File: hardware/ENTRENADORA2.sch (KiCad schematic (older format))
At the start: 74 parts

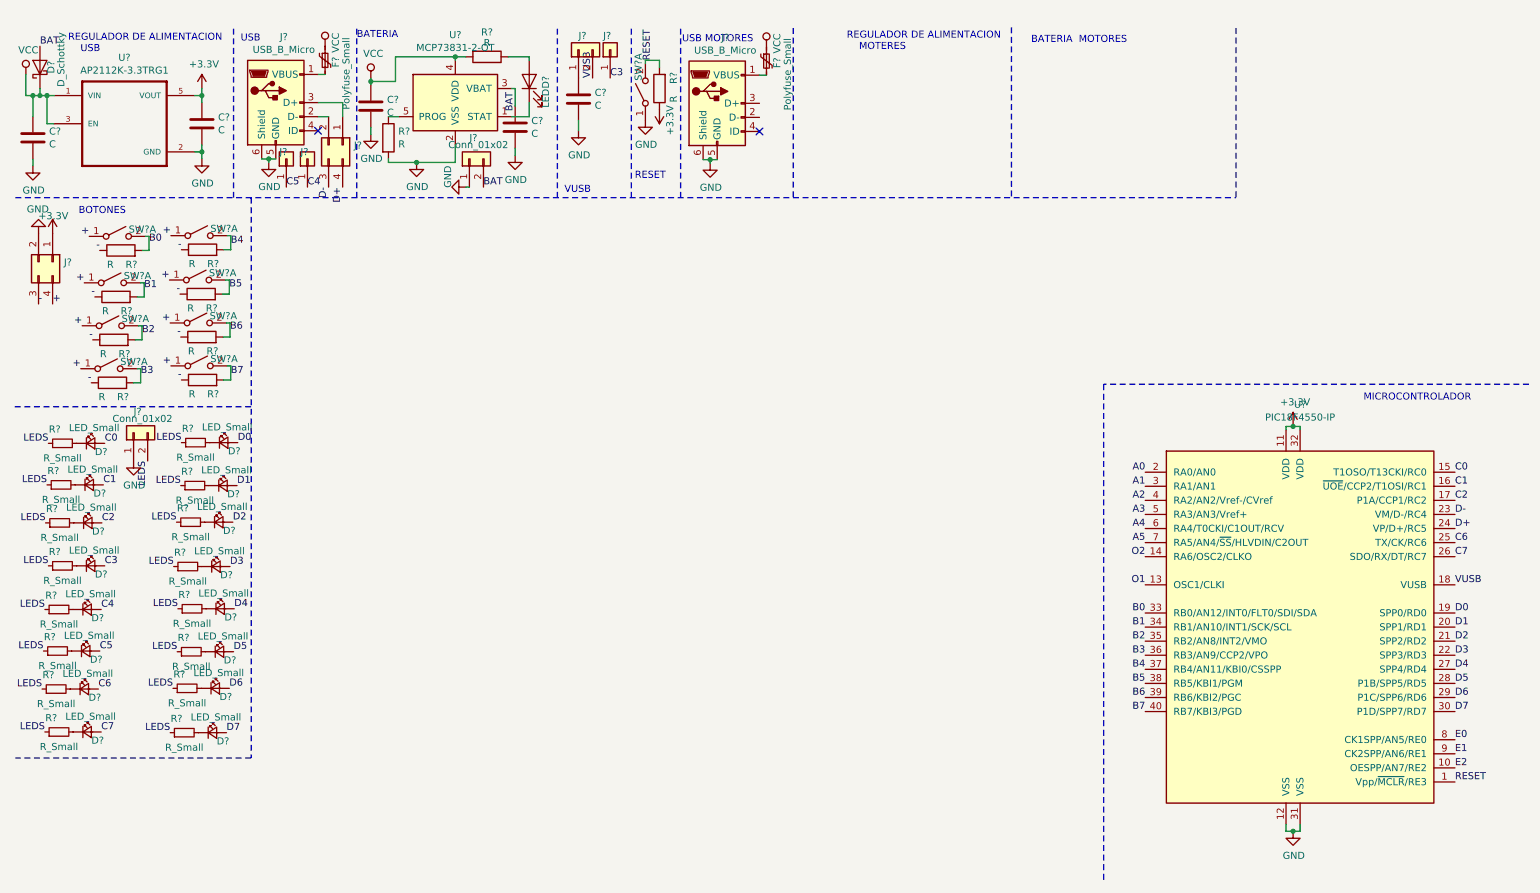
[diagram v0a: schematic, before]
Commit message: co
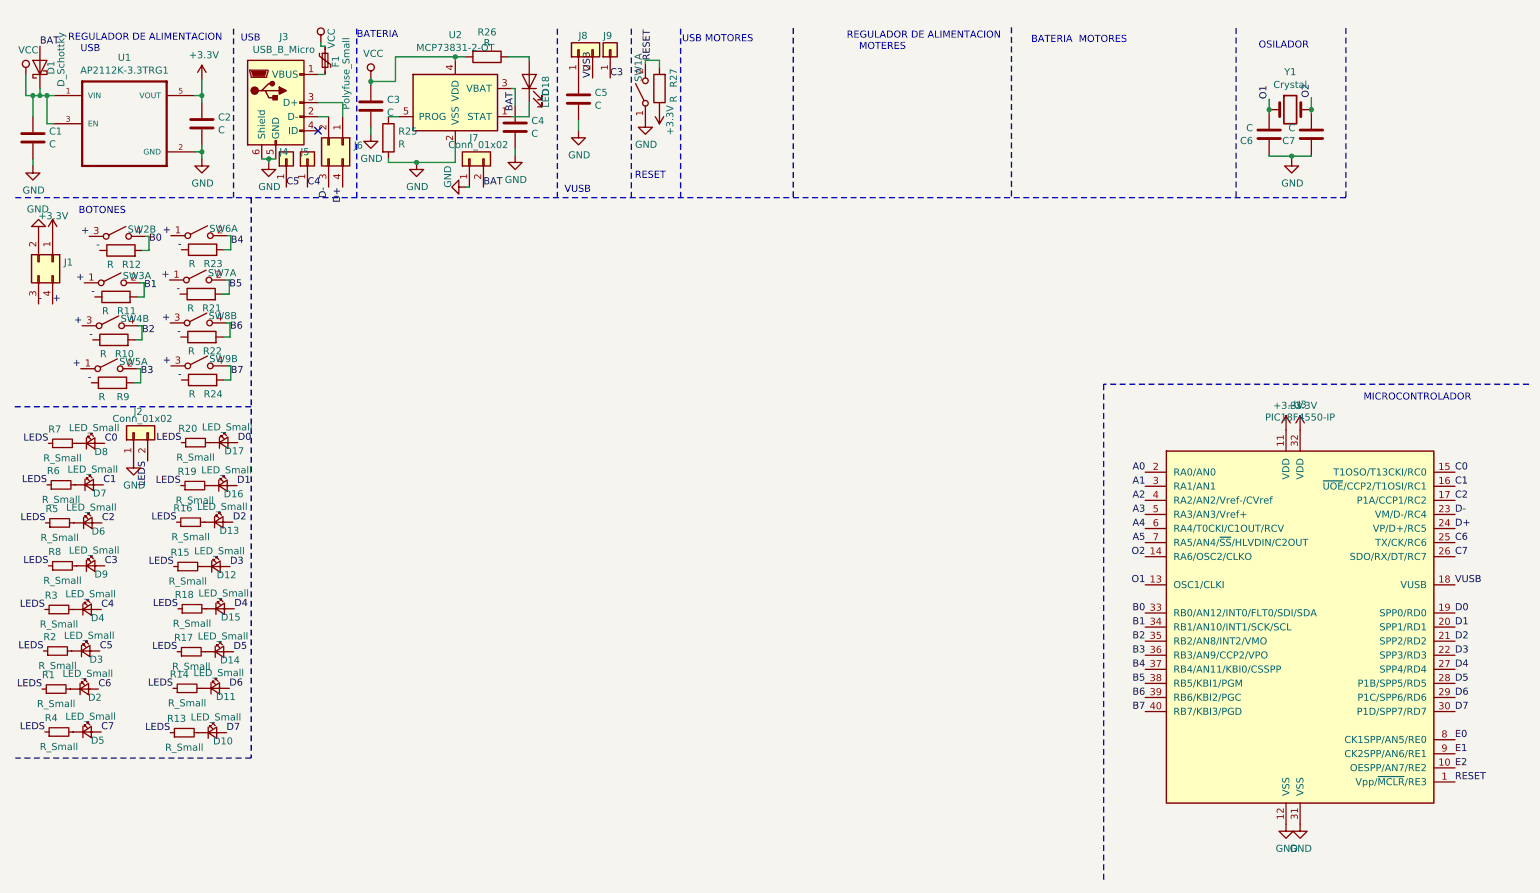
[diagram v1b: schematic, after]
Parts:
- removed F?: Polyfuse_Small, symbol Device:Polyfuse_Small
- removed J?: USB_B_Micro, symbol Connector:USB_B_Micro
- added C6, C7: C, Capacitor_SMD:C_0805_2012Metric_Pad1.15x1.40mm_HandSolder, symbol Device:C
- added Y1: Crystal, Crystal:Crystal_HC49-U_Vertical, symbol Device:Crystal
- C1, C2, C3, C4, C5: renamed from C?; footprint (none) -> Capacitor_SMD:C_0805_2012Metric_Pad1.15x1.40mm_HandSolder
- D1: renamed from D?; footprint (none) -> Diode_SMD:D_SOD-123
- D10, D11, D12, D13, D14, D15, D16, D17, D18, D2, D3, D4, D5, D6, D7, D8, D9: renamed from D?; footprint (none) -> LED_SMD:LED_0805_2012Metric_Pad1.15x1.40mm_HandSolder
- F1: renamed from F?; footprint (none) -> Fuse:Fuse_0805_2012Metric_Pad1.15x1.40mm_HandSolder
- J1, J6: renamed from J?; footprint (none) -> Connector_PinHeader_2.54mm:PinHeader_2x02_P2.54mm_Vertical
- J2, J7, J8: renamed from J?; footprint (none) -> Connector_PinHeader_2.54mm:PinHeader_1x02_P2.54mm_Vertical
- J3: renamed from J?; footprint (none) -> Connectors_EC:629105150521
- J4, J5, J9: renamed from J?; footprint (none) -> Connector_PinHeader_2.54mm:PinHeader_1x01_P2.54mm_Vertical
- R1, R10, R11, R12, R13, R14, R15, R16, R17, R18, R19, R2, R20, R21, R22, R23, R24, R25, R26, R27, R3, R4, R5, R6, R7, R8, R9: renamed from R?; footprint (none) -> Resistor_SMD:R_0805_2012Metric_Pad1.15x1.40mm_HandSolder
- SW1, SW2, SW3, SW4, SW5, SW6, SW7, SW8, SW9: renamed from SW?; footprint (none) -> Button_Switch_SMD:SW_SPST_TL3342
- U1: renamed from U?; footprint SOT95P285X140-5N -> Package_TO_SOT_SMD:SOT-23-5
- gave numbers to parts that had none: 2
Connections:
- net +: now also SW2.3 (A), SW4.3 (A), SW8.3 (A), SW9.3 (A); no longer SW2.1 (A), SW4.1 (A), SW8.1 (A), SW9.1 (A)
- net B0: now also SW2.4 (B); no longer SW2.2 (B)
- net B2: now also SW4.4 (B); no longer SW4.2 (B)
- net B6: now also SW8.4 (B); no longer SW8.2 (B)
- net B7: now also SW9.4 (B); no longer SW9.2 (B)
- net GND: now also C6.1, C7.1
- net O1: now also C6.2, Y1.1
- net O2: now also C7.2, Y1.2
- no-connect marks 2 -> 1
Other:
- note added: "OSILADOR"
